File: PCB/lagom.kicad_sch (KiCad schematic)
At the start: 154 parts

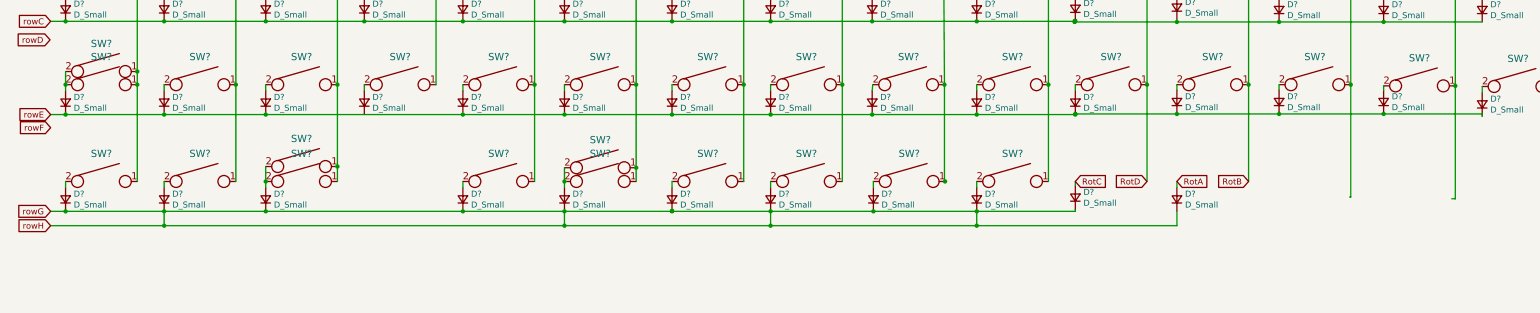
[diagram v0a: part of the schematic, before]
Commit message: Matrix almost done
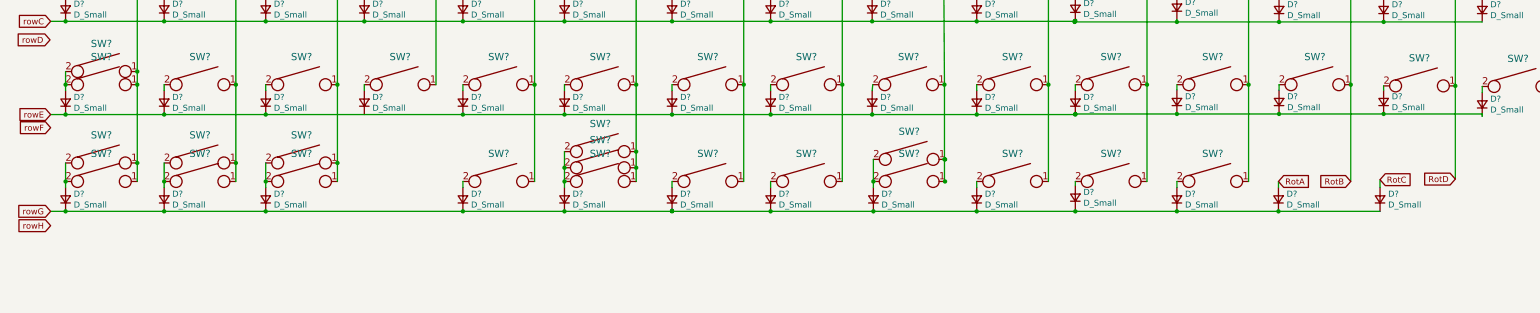
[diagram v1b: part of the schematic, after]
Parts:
- added D? (x2): D_Small, Keebio-Parts:Diode, symbol Device:D_Small
- added SW?: KEYSW, Button_Switch_Keyboard:SW_Cherry_MX_7u_PCB, symbol keyboard_parts:KEYSW
- added SW? (x2): KEYSW, Button_Switch_Keyboard:SW_Cherry_MX_1.00u_PCB, symbol keyboard_parts:KEYSW
- added SW?: KEYSW, Button_Switch_Keyboard:SW_Cherry_MX_1.50u_PCB, symbol keyboard_parts:KEYSW
- added SW? (x2): KEYSW, Button_Switch_Keyboard:SW_Cherry_MX_1.25u_PCB, symbol keyboard_parts:KEYSW
- SW?: footprint Button_Switch_Keyboard:SW_Cherry_MX_1.25u_PCB -> Button_Switch_Keyboard:SW_Cherry_MX_1.50u_PCB
- SW? (x2): footprint Button_Switch_Keyboard:SW_Cherry_MX_1.00u_PCB -> Button_Switch_Keyboard:SW_Cherry_MX_1.25u_PCB
- SW?: footprint Button_Switch_Keyboard:SW_Cherry_MX_1.00u_PCB -> Button_Switch_Keyboard:SW_Cherry_MX_1.50u_PCB
- SW?: footprint Button_Switch_Keyboard:SW_Cherry_MX_1.25u_PCB -> Button_Switch_Keyboard:SW_Cherry_MX_1.00u_PCB
- SW?: footprint Button_Switch_Keyboard:SW_Cherry_MX_1.25u_PCB -> Button_Switch_Keyboard:SW_Cherry_MX_ISOEnter_PCB
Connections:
- net RotA: now also D?.2 (A); no longer D?.2 (A)
- net RotB: now also SW?.1, SW?.1, SW?.1, SW?.1; no longer SW?.1, SW?.1, SW?.1, SW?.1
- net RotC: now also D?.2 (A); no longer D?.2 (A)
- net RotD: now also SW?.1, SW?.1, SW?.1, SW?.1, SW?.1; no longer SW?.1, SW?.1, SW?.1, SW?.1
- net rowG: now also D?.1 (K), D?.1 (K); no longer U?.20 (A3/PF4)
- net at SW?.1, SW?.1, SW?.1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: now also SW?.1 (x2)
- net at SW?.1, SW?.1, SW?.1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: now also SW?.1
- net at D?.2 (A), SW?.2: now also SW?.2 (x3)
- net at SW?.1, SW?.1, SW?.1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: now also SW?.1
- net at D?.2 (A), SW?.2, SW?.2: now also SW?.2
- new net: SW?.1, SW?.1, SW?.1, SW?.1, SW?.1 (x2)
- new net: D?.2 (A), SW?.2 (x2)
- new net rowH: U?.20 (A3/PF4)
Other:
- moved on the sheet: SW?
